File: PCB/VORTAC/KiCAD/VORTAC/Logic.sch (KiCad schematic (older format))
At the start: 17 parts, among them IC1 TMC2209-LA-T, Q1 WSD4066DN, Q2 WSD4066DN, Q3 WSD4066DN

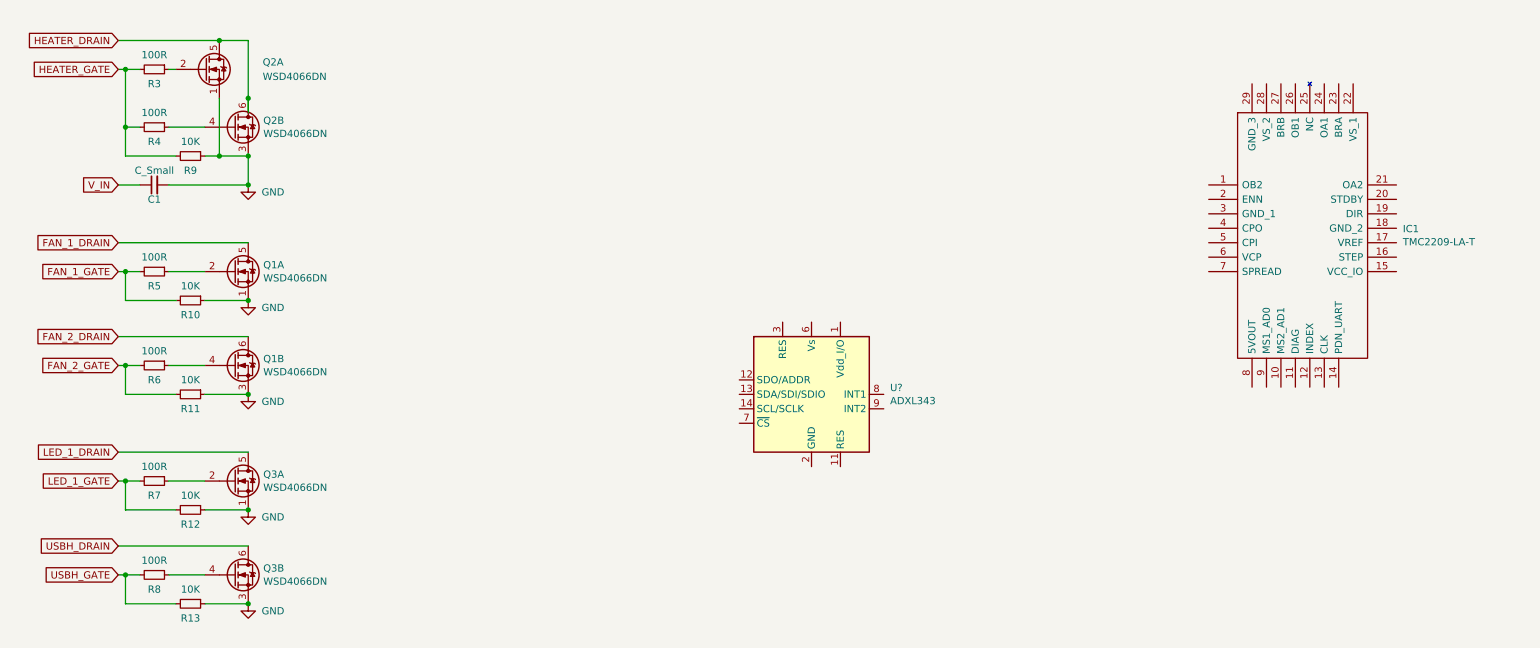
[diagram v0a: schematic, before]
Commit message: TMC and Acc preperation
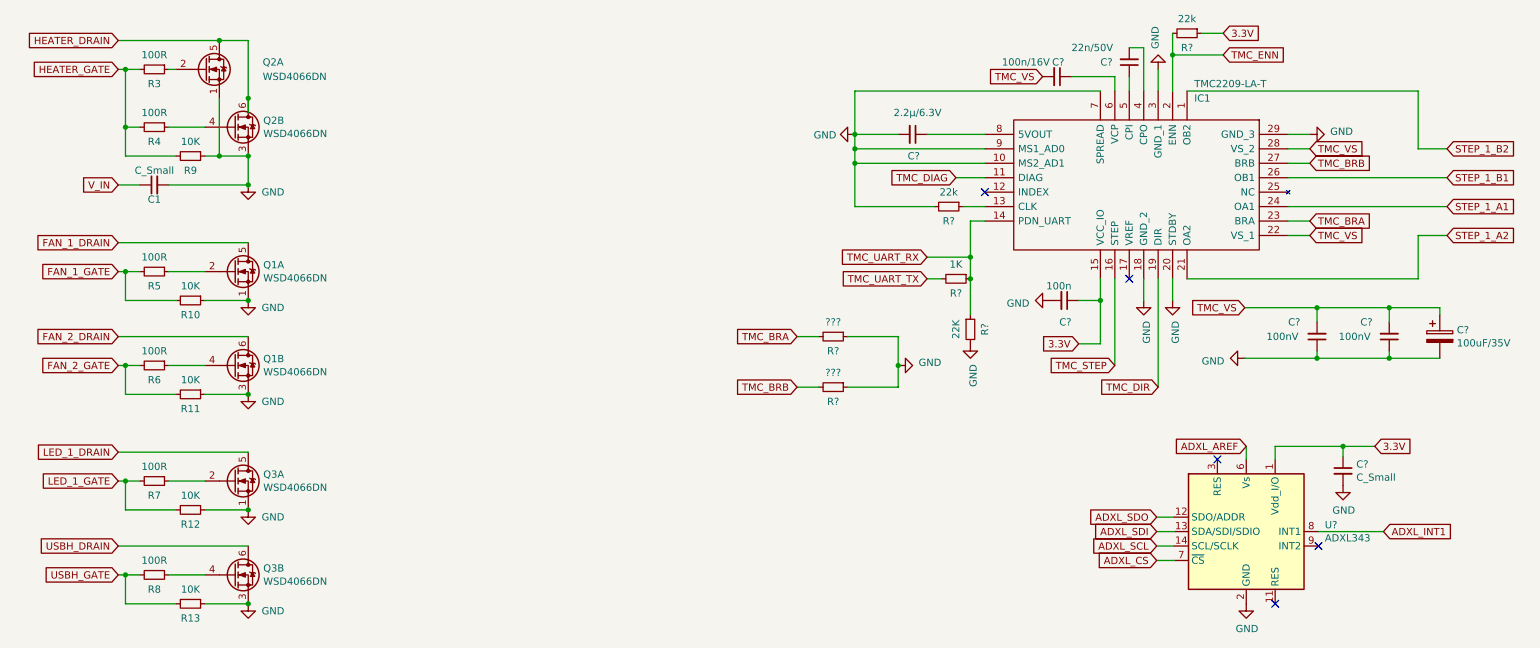
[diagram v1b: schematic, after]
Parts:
- added C?: C_Small, symbol Device:C_Small
- added C?: 22n/50V, symbol Device:C_Small
- added C?: 100n/16V, symbol Device:C_Small
- added C?: 2.2μ/6.3V, symbol Device:C_Small
- added C? (x2): 100nV, symbol Device:C_Small
- added C?: 100uF/35V, symbol Device:CP
- added C?: 100n, symbol Device:C_Small
- added R? (x2): 22k, symbol Device:R_Small
- added R?: 22K, symbol Device:R_Small
- added R?: 1K, symbol Device:R_Small
- added R? (x2): ???, symbol Device:R_Small
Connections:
- net GND: now also IC1.10 (MS2_AD1), IC1.18 (GND_2), IC1.20 (STDBY), IC1.29 (GND_3), IC1.3 (GND_1), IC1.7 (SPREAD), IC1.9 (MS1_AD0), U?.2 (GND), U?.4 (GND), U?.5 (GND), C?.1, C?.1, C?.2, C?.2, C?.2, C?.2, R?.1, R?.1, R?.2, R?.2
- net STEP_1_B2: now reaches IC1.1 (OB2)
- net TMC_DIAG: now reaches IC1.11 (DIAG)
- net at IC1.13 (CLK): now also R?.1
- net TMC_UART_RX: now reaches IC1.14 (PDN_UART)
- net TMC_UART_RX: now also R?.1, R?.1
- net 3.3V: now reaches IC1.15 (VCC_IO)
- net 3.3V: now also U?.1 (Vdd_I/O), C?.1, C?.1, R?.1
- net TMC_STEP: now reaches IC1.16 (STEP)
- net TMC_DIR: now reaches IC1.19 (DIR)
- net TMC_ENN: now reaches IC1.2 (ENN)
- net TMC_ENN: now also R?.2
- net STEP_1_A2: now reaches IC1.21 (OA2)
- net TMC_VS: now reaches IC1.22 (VS_1)
- net TMC_VS: now also IC1.28 (VS_2), C?.1, C?.2, C?.2, C?.2
- net TMC_BRA: now reaches IC1.23 (BRA)
- net TMC_BRA: now also R?.2
- net STEP_1_A1: now reaches IC1.24 (OA1)
- net STEP_1_B1: now reaches IC1.26 (OB1)
- net TMC_BRB: now reaches IC1.27 (BRB)
- net TMC_BRB: now also R?.2
- net at IC1.4 (CPO): now also C?.2
- net at IC1.5 (CPI): now also C?.1
- net at IC1.6 (VCP): now also C?.1
- net at IC1.8 (5VOUT): now also C?.1
- net ADXL_SDO: now reaches U?.12 (SDO/ADDR)
- net ADXL_SDI: now reaches U?.13 (SDA/SDI/SDIO)
- net ADXL_SCL: now reaches U?.14 (SCL/SCLK)
- net ADXL_AREF: now reaches U?.6 (Vs)
- net ADXL_CS: now reaches U?.7 (~CS)
- net ADXL_INT1: now reaches U?.8 (INT1)
- new net TMC_UART_TX: R?.2
- no-connect marks 0 -> 5
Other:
- moved on the sheet: IC1, U?
